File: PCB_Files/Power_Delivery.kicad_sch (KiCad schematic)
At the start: 8 parts, among them SW2 SW_SPST, U4 SPX1117M3-L-3-3/TR

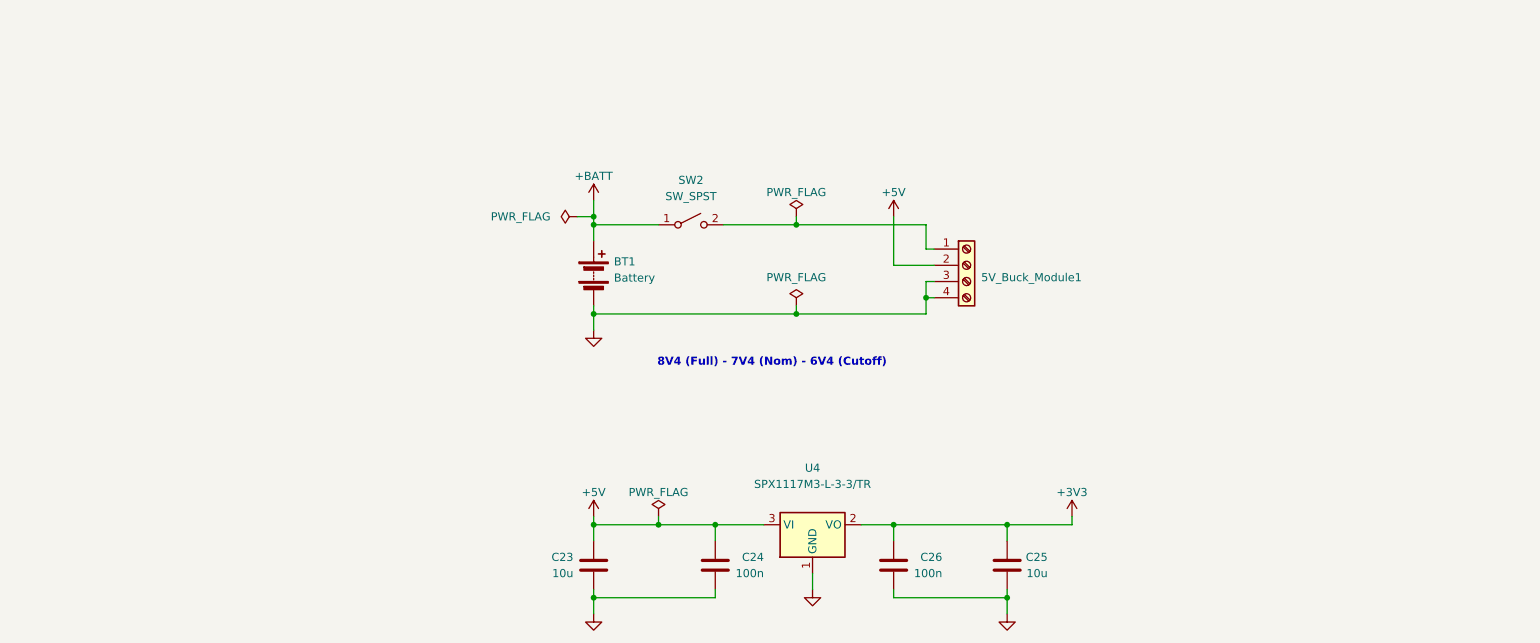
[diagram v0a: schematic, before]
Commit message: General schematic clean up and footprint allocation.
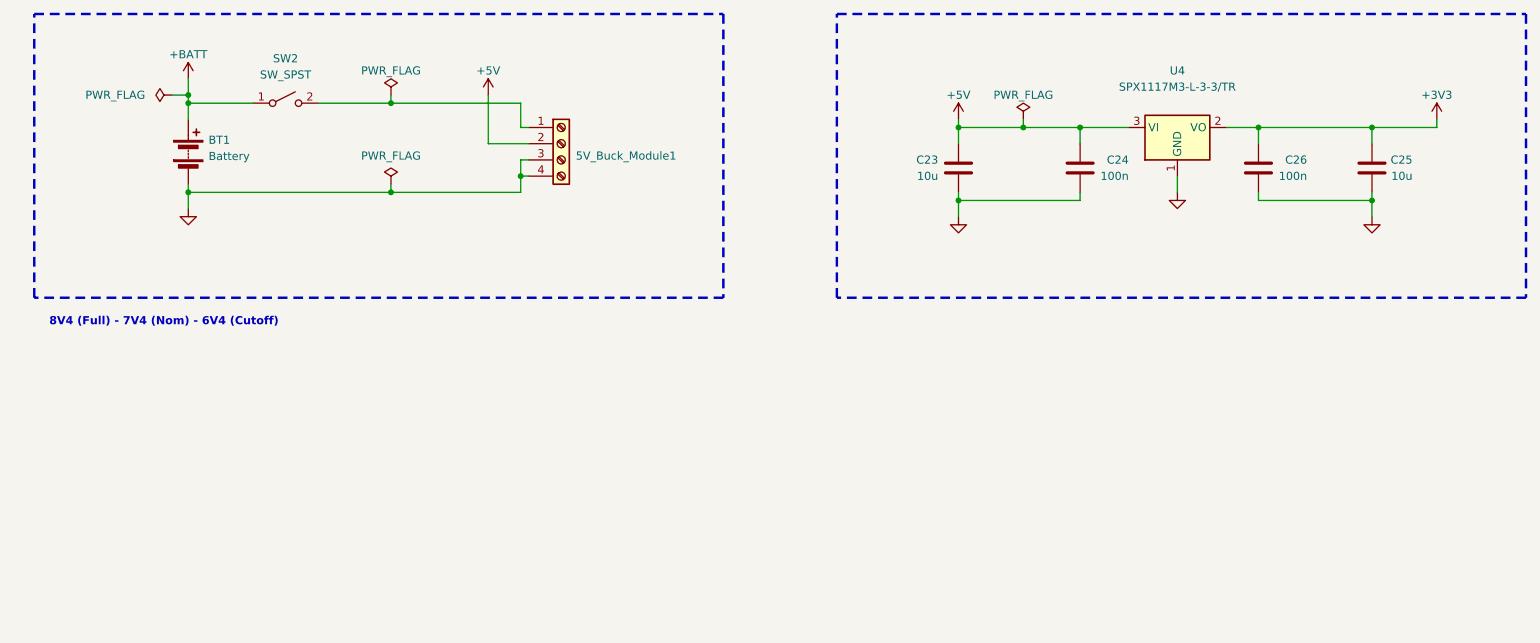
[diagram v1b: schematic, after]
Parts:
- C23, C24, C25, C26: footprint (none) -> Capacitor_SMD:C_0603_1608Metric
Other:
- moved on the sheet: 5V_Buck_Module1, BT1, C23, C24, C25, C26, SW2, U4
